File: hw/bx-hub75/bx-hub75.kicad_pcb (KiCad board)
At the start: 2 copper layers, 63.5 x 50.8 mm, 17 parts, among them J1 DB9_Male, J2 Barrel_Jack_MountingPin, U1 74HCT541, U2 74HCT541, U3 LD1117S33TR_SOT223

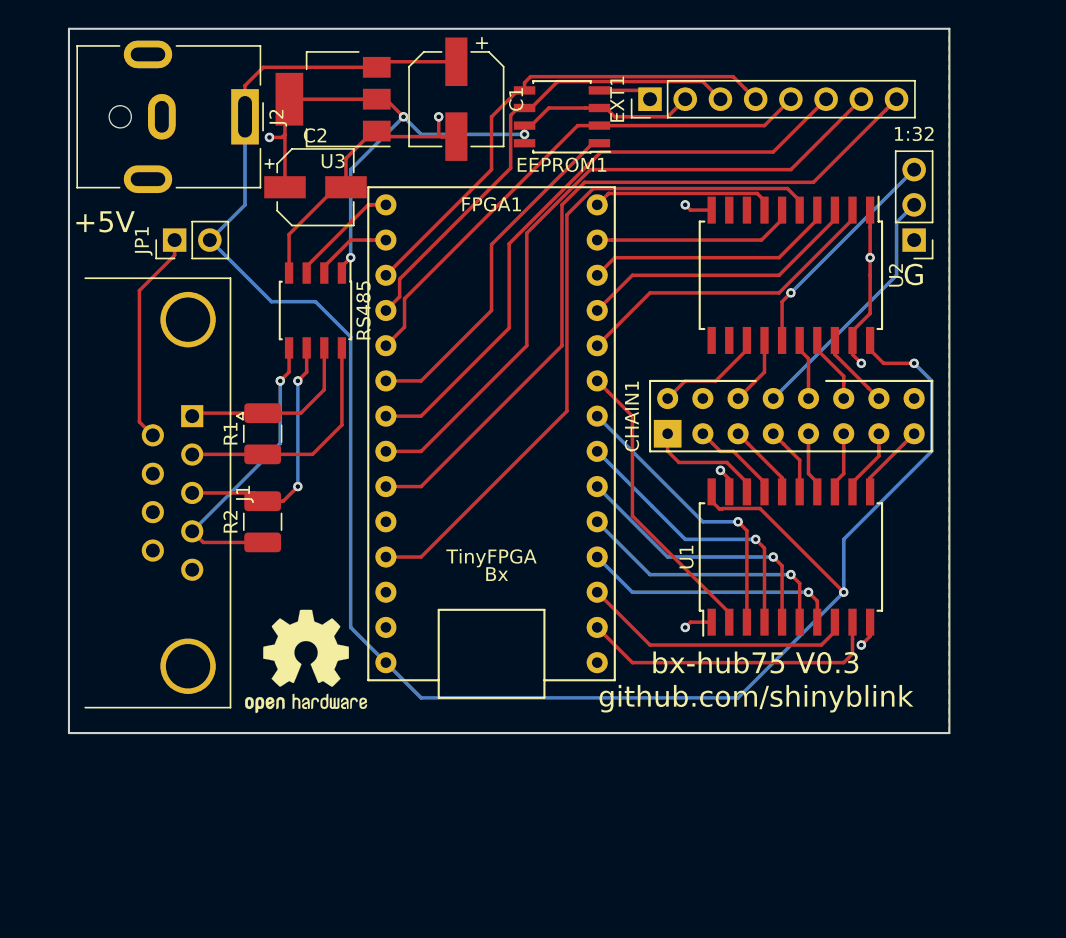
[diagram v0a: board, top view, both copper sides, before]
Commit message: hw/bx-hub75: release V0.4.
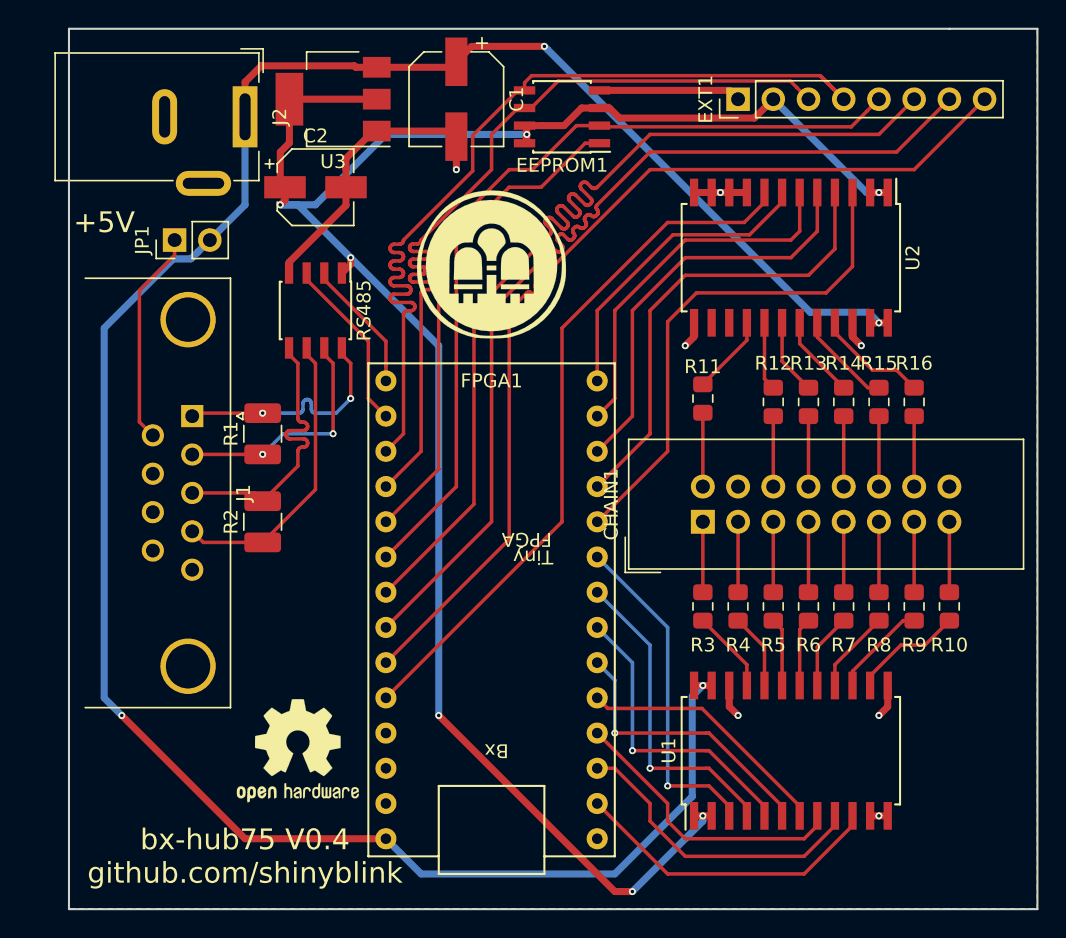
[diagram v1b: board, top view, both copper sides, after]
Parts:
- removed 1:32: E Line Enable, Connector_PinHeader_2.54mm:PinHeader_1x03_P2.54mm_Vertical
- added G***: LOGO, Random:shinyblink_1x1cm, F.Cu at (68.6, 80.6)
- added R10: 33, Resistor_SMD:R_0805_2012Metric_Pad1.15x1.40mm_HandSolder, F.Cu at (101.6, 105.2)
- added R11: 33, Resistor_SMD:R_0805_2012Metric_Pad1.15x1.40mm_HandSolder, F.Cu at (83.8, 90.2)
- added R12: 33, Resistor_SMD:R_0805_2012Metric_Pad1.15x1.40mm_HandSolder, F.Cu at (88.9, 90.4)
- added R13: 33, Resistor_SMD:R_0805_2012Metric_Pad1.15x1.40mm_HandSolder, F.Cu at (91.4, 90.4)
- added R14: 33, Resistor_SMD:R_0805_2012Metric_Pad1.15x1.40mm_HandSolder, F.Cu at (94.0, 90.4)
- added R15: 33, Resistor_SMD:R_0805_2012Metric_Pad1.15x1.40mm_HandSolder, F.Cu at (96.5, 90.4)
- added R16: 33, Resistor_SMD:R_0805_2012Metric_Pad1.15x1.40mm_HandSolder, F.Cu at (99.1, 90.4)
- added R3: 33, Resistor_SMD:R_0805_2012Metric_Pad1.15x1.40mm_HandSolder, F.Cu at (83.8, 105.2)
- added R4: 33, Resistor_SMD:R_0805_2012Metric_Pad1.15x1.40mm_HandSolder, F.Cu at (86.4, 105.2)
- added R5: 33, Resistor_SMD:R_0805_2012Metric_Pad1.15x1.40mm_HandSolder, F.Cu at (88.9, 105.2)
- added R6: 33, Resistor_SMD:R_0805_2012Metric_Pad1.15x1.40mm_HandSolder, F.Cu at (91.4, 105.2)
- added R7: 33, Resistor_SMD:R_0805_2012Metric_Pad1.15x1.40mm_HandSolder, F.Cu at (94.0, 105.2)
- added R8: 33, Resistor_SMD:R_0805_2012Metric_Pad1.15x1.40mm_HandSolder, F.Cu at (96.5, 105.2)
- added R9: 33, Resistor_SMD:R_0805_2012Metric_Pad1.15x1.40mm_HandSolder, F.Cu at (99.1, 105.2)
- CHAIN1: footprint Random:HUB75_HEADER -> Connector_IDC:IDC-Header_2x08_P2.54mm_Vertical
- J2: value Barrel_Jack_MountingPin -> Barrel_Jack; footprint Connector_BarrelJack:BarrelJack_CUI_PJ-063AH_Horizontal -> Connector_BarrelJack:BarrelJack_Wuerth_6941xx301002
- U1, U2: value 74HCT541 -> 74LVC4245A; footprint Package_SO:SOIC-20W_7.5x12.8mm_P1.27mm -> Package_SO:SOIC-24W_7.5x15.4mm_P1.27mm
- moved U1 14.0 mm to (90.2, 115.6)
- moved FPGA1 12.7 mm to (68.6, 104.1)
- moved CHAIN1 9.92 mm to (83.8, 99.1), turned to 90 degrees
- moved OSHW1 6.47 mm to (54.6, 115.6)
- moved EXT1 6.35 mm to (86.4, 68.6)
- moved U2 1.27 mm to (90.2, 80.0)
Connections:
- CHAIN1 pad 8: /E_PIN -> Net-(CHAIN1-Pad8)
- FPGA1 pad 13: /G2 -> /E
- FPGA1 pad 14: /G1 -> /G2
- FPGA1 pad 15: /TX -> /RX
- FPGA1 pad 16: /RX -> /TX
- FPGA1 pad 24: Net-(FPGA1-Pad24) -> /G1
- FPGA1 pad 25: /E -> Net-(FPGA1-Pad25)
- J1 pad 1: /RX- -> /RX+
- J1 pad 2: /RX+ -> /RX-
- R1 pad 1: /RX+ -> /RX-
- R1 pad 2: /RX- -> /RX+
- RS485 pad 5: /TX- -> /TX+
- RS485 pad 6: /TX+ -> /TX-
- U1 pad 1: GND -> +3V3
- U1 pad 10: GND -> /OE
- U1 pad 11: Net-(CHAIN1-Pad15) -> GND
- U1 pad 12: Net-(CHAIN1-Pad13) -> GND
- U1 pad 13: Net-(CHAIN1-Pad11) -> GND
- U1 pad 14: Net-(CHAIN1-Pad9) -> Net-(R10-Pad2)
- U1 pad 15: Net-(CHAIN1-Pad7) -> Net-(R9-Pad2)
- U1 pad 16: Net-(CHAIN1-Pad5) -> Net-(R8-Pad2)
- U1 pad 17: Net-(CHAIN1-Pad3) -> Net-(R7-Pad2)
- U1 pad 18: Net-(CHAIN1-Pad1) -> Net-(R6-Pad2)
- U1 pad 19: GND -> Net-(R5-Pad2)
- U1 pad 2: /R1 -> +3V3
- U1 pad 20: +5V -> Net-(R4-Pad2)
- U1 pad 3: /B1 -> /R1
- U1 pad 4: /R2 -> /B1
- U1 pad 5: /B2 -> /R2
- U1 pad 6: /A -> /B2
- U1 pad 7: /C -> /A
- U1 pad 8: /CLK -> /C
- U1 pad 9: /OE -> /CLK
- U2 pad 1: GND -> +3V3
- U2 pad 11: Net-(U2-Pad11) -> GND
- U2 pad 12: Net-(U2-Pad12) -> GND
- U2 pad 13: Net-(CHAIN1-Pad2) -> GND
- U2 pad 14: Net-(CHAIN1-Pad6) -> Net-(U2-Pad14)
- U2 pad 15: /E_DRV -> Net-(U2-Pad15)
- U2 pad 16: Net-(CHAIN1-Pad10) -> Net-(R11-Pad1)
- U2 pad 17: Net-(CHAIN1-Pad12) -> Net-(R12-Pad1)
- U2 pad 18: Net-(CHAIN1-Pad14) -> Net-(R13-Pad1)
- U2 pad 19: GND -> Net-(R14-Pad1)
- U2 pad 2: /LAT -> +3V3
- U2 pad 20: +5V -> Net-(R15-Pad1)
- U2 pad 3: /D -> /LAT
- U2 pad 4: /B -> /D
- U2 pad 5: /E -> /B
- U2 pad 6: /G2 -> /E
- U2 pad 7: /G1 -> /G2
- U2 pad 8: Net-(U2-Pad8) -> /G1
- U2 pad 9: Net-(U2-Pad9) -> GND
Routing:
- net +3V3: track 53.0 -> 139.8 mm, vias 4 -> 7
- net /G1: track 13.3 -> 51.0 mm
- net /MOSI: track 35.8 -> 65.4 mm
- net /SCK: track 34.5 -> 60.4 mm
- net /SC_EXT: track 44.8 -> 70.1 mm
- net +5V: track 140.4 -> 165.4 mm, vias 2 -> 4
- net /E: track 50.2 -> 26.6 mm
- net /MISO: track 38.2 -> 59.6 mm
- net /EXT_IO1: track 49.6 -> 70.0 mm
- net /E_PIN: track 18.2 -> 0.00 mm
- net /E_DRV: track 16.3 -> 0.00 mm, vias 1 -> 0
- net /EXT_IO2: track 54.4 -> 70.2 mm
- net /LAT: track 22.9 -> 36.9 mm
- net /D: track 20.5 -> 34.2 mm
- net /CS_EEPROM: track 25.3 -> 38.7 mm
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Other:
- board size 63.5 x 50.8 mm -> 69.8 x 63.5 mm
- net class Default: clearance 0.1 -> 0.127; via_dia 0.6858 -> 0.508; via_drill 0.3302 -> 0.254
- net class Power added: clearance 0.254, trace_width 0.508, via_dia 0.508, via_drill 0.254
- rule trace_clearance: 0.1 -> 0.127
- rule trace_min: 0.1524 -> 0.127
- rule via_min_drill: 0.3302 -> 0.254
- rule via_min_size: 0.6858 -> 0.508
- board text added: "bx-hub75 V0.4 github.com/shinyblink"
- board text removed: "G"
- board text removed: "bx-hub75 V0.3 github.com/shinyblink"
